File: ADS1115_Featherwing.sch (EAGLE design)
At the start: 25 parts, among them J1 4P-SMD-2.0-90D, J2 ST-PJ-312, U1 ADS1115IDGST

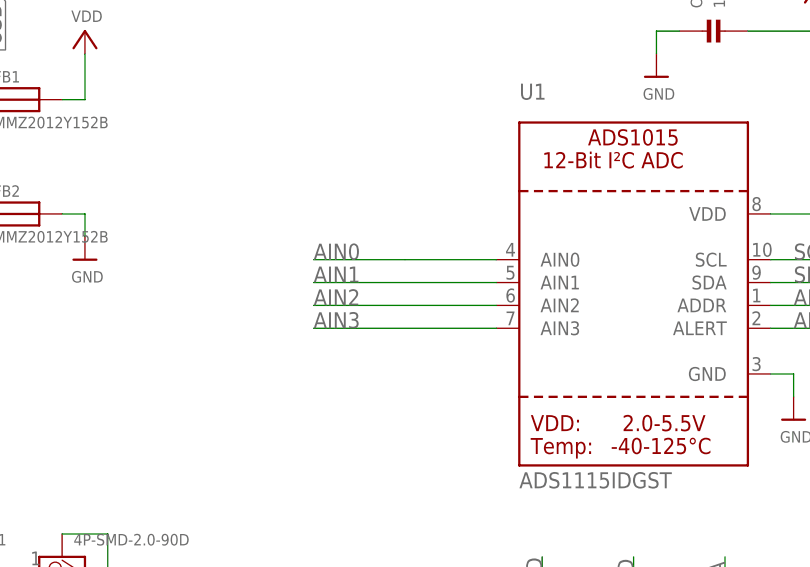
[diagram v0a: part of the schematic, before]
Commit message: Added protection resistor
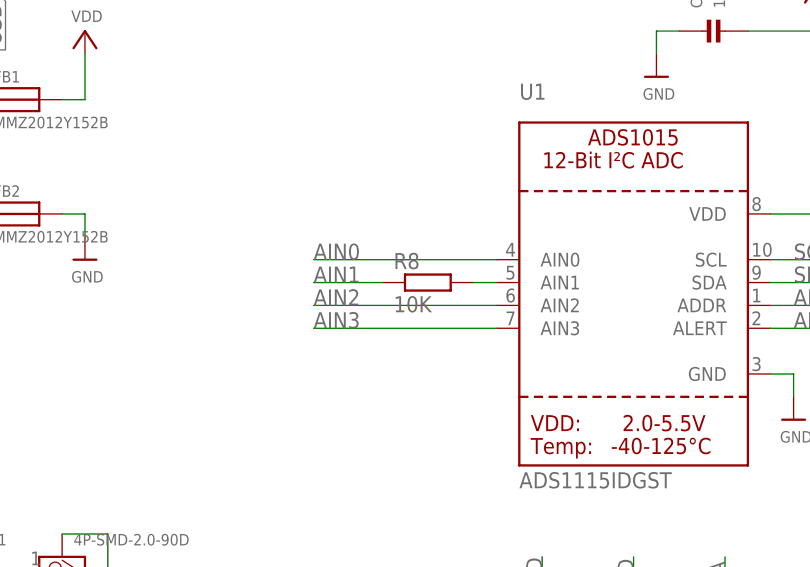
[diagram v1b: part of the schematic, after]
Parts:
- added R8: 10K, resistor:R-EU_R0603
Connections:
- new net N$1: R8.2, U1.AIN1
- net AIN1: now also R8.1; no longer U1.AIN1
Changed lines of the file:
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@@
 <?xml version="1.0" encoding="utf-8"?>
 <!DOCTYPE eagle SYSTEM "eagle.dtd">
-<eagle version="7.1.0">
+<eagle version="7.4.0">
 <drawing>
 <settings>
@@
 <grid distance="0.1" unitdist="inch" unit="inch" style="lines" multiple="1" display="no" altdistance="0.01" altunitdist="inch" altunit="inch"/>
 <layers>
-<layer number="1" name="Top" color="4" fill="1" visible="yes" active="no"/>
-<layer number="16" name="Bottom" color="1" fill="1" visible="yes" active="no"/>
-<layer number="17" name="Pads" color="2" fill="1" visible="yes" active="no"/>
-<layer number="18" name="Vias" color="2" fill="1" visible="yes" active="no"/>
-<layer number="19" name="Unrouted" color="6" fill="1" visible="yes" active="no"/>
-<layer number="20" name="Dimension" color="15" fill="1" visible="yes" active="no"/>
-<layer number="21" name="tPlace" color="7" fill="1" visible="yes" active="no"/>
-<layer number="22" name="bPlace" color="11" fill="1" visible="yes" active="no"/>
-<layer number="23" name="tOrigins" color="15" fill="1" visible="yes" active="no"/>
-<layer number="24" name="bOrigins" color="15" fill="1" visible="yes" active="no"/>
-<layer number="25" name="tNames" color="7" fill="1" visible="yes" active="no"/>
-<layer number="26" name="bNames" color="11" fill="1" visible="yes" active="no"/>
-<layer number="27" name="tValues" color="7" fill="1" visible="yes" active="no"/>
-<layer number="28" name="bValues" color="7" fill="1" visible="yes" active="no"/>
+<layer number="1" name="Top" color="4" fill="1" visible="no" active="no"/>
+<layer number="16" name="Bottom" color="1" fill="1" visible="no" active="no"/>
+<layer number="17" name="Pads" color="2" fill="1" visible="no" active="no"/>
+<layer number="18" name="Vias" color="2" fill="1" visible="no" active="no"/>
+<layer number="19" name="Unrouted" color="6" fill="1" visible="no" active="no"/>
+<layer number="20" name="Dimension" color="15" fill="1" visible="no" active="no"/>
+<layer number="21" name="tPlace" color="7" fill="1" visible="no" active="no"/>
+<layer number="22" name="bPlace" color="11" fill="1" visible="no" active="no"/>
+<layer number="23" name="tOrigins" color="15" fill="1" visible="no" active="no"/>
+<layer number="24" name="bOrigins" color="15" fill="1" visible="no" active="no"/>
+<layer number="25" name="tNames" color="7" fill="1" visible="no" active="no"/>
+<layer number="26" name="bNames" color="11" fill="1" visible="no" active="no"/>
+<layer number="27" name="tValues" color="7" fill="1" visible="no" active="no"/>
+<layer number="28" name="bValues" color="7" fill="1" visible="no" active="no"/>
 <layer number="29" name="tStop" color="7" fill="3" visible="no" active="no"/>
 <layer number="30" name="bStop" color="7" fill="6" visible="no" active="no"/>
@@
 <layer number="35" name="tGlue" color="7" fill="4" visible="no" active="no"/>
 <layer number="36" name="bGlue" color="7" fill="5" visible="no" active="no"/>
-<layer number="37" name="tTest" color="7" fill="1" visible="yes" active="no"/>
-<layer number="38" name="bTest" color="7" fill="1" visible="yes" active="no"/>
+<layer number="37" name="tTest" color="7" fill="1" visible="no" active="no"/>
+<layer number="38" name="bTest" color="7" fill="1" visible="no" active="no"/>
 <layer number="39" name="tKeepout" color="4" fill="11" visible="no" active="no"/>
 <layer number="40" name="bKeepout" color="1" fill="11" visible="no" active="no"/>
@@
 <layer number="44" name="Drills" color="7" fill="1" visible="no" active="no"/>
 <layer number="45" name="Holes" color="7" fill="1" visible="no" active="no"/>
-<layer number="46" name="Milling" color="3" fill="1" visible="yes" active="no"/>
-<layer number="47" name="Measures" color="7" fill="1" visible="yes" active="no"/>
-<layer number="48" name="Document" color="7" fill="1" visible="yes" active="no"/>
-<layer number="49" name="Reference" color="7" fill="1" visible="yes" active="no"/>
-<layer number="50" name="dxf" color="7" fill="1" visible="yes" active="no"/>
-<layer number="51" name="tDocu" color="7" fill="1" visible="yes" active="no"/>
-<layer number="52" name="bDocu" color="7" fill="1" visible="yes" active="no"/>
-<layer number="53" name="tGND_GNDA" color="7" fill="9" visible="yes" active="no"/>
-<layer number="54" name="bGND_GNDA" color="1" fill="9" visible="yes" active="no"/>
-<layer number="56" name="wert" color="7" fill="1" visible="yes" active="no"/>
-<layer number="57" name="tCAD" color="7" fill="1" visible="yes" active="no"/>
-<layer number="59" name="tCarbon" color="7" fill="1" visible="yes" active="no"/>
-<layer number="60" name="bCarbon" color="7" fill="1" visible="yes" active="no"/>
+<layer number="46" name="Milling" color="3" fill="1" visible="no" active="no"/>
+<layer number="47" name="Measures" color="7" fill="1" visible="no" active="no"/>
+<layer number="48" name="Document" color="7" fill="1" visible="no" active="no"/>
+<layer number="49" name="Reference" color="7" fill="1" visible="no" active="no"/>
+<layer number="50" name="dxf" color="7" fill="1" visible="no" active="no"/>
+<layer number="51" name="tDocu" color="7" fill="1" visible="no" active="no"/>
+<layer number="52" name="bDocu" color="7" fill="1" visible="no" active="no"/>
+<layer number="53" name="tGND_GNDA" color="7" fill="9" visible="no" active="no"/>
+<layer number="54" name="bGND_GNDA" color="1" fill="9" visible="no" active="no"/>
+<layer number="56" name="wert" color="7" fill="1" visible="no" active="no"/>
+<layer number="57" name="tCAD" color="7" fill="1" visible="no" active="no"/>
+<layer number="59" name="tCarbon" color="7" fill="1" visible="no" active="no"/>
+<layer number="60" name="bCarbon" color="7" fill="1" visible="no" active="no"/>
 <layer number="90" name="Modules" color="5" fill="1" visible="yes" active="yes"/>
 <layer number="91" name="Nets" color="2" fill="1" visible="yes" active="yes"/>
@@
 <part name="J1" library="Seeed-OPL-Connector" deviceset="GROVE-CONNECTOR-SMD-90D(4+2P-2.0)" device="" value="4P-SMD-2.0-90D"/>
 <part name="C5" library="adafruit" deviceset="CPOL-US" device="153CLV-0810" value="100uF 50V"/>
+<part name="R8" library="resistor" deviceset="R-EU_" device="R0603" value="10K"/>
 </parts>
 <sheets>
@@
 <instance part="J1" gate="G$1" x="-12.7" y="7.62"/>
 <instance part="C5" gate="G$1" x="101.6" y="114.3"/>
+<instance part="R8" gate="G$1" x="27.94" y="43.18"/>
 </instances>
 <busses>
@@
 <net name="AIN0" class="1">
 <segment>
+<label x="15.24" y="45.72" size="1.778" layer="95"/>
+<wire x1="15.24" y1="45.72" x2="35.56" y2="45.72" width="0.1524" layer="91"/>
 <pinref part="U1" gate="G$1" pin="AIN0"/>
-<wire x1="35.56" y1="45.72" x2="25.4" y2="45.72" width="0.1524" layer="91"/>
-<label x="15.24" y="45.72" size="1.778" layer="95"/>
-<wire x1="25.4" y1="45.72" x2="15.24" y2="45.72" width="0.1524" layer="91"/>
 </segment>
 <segment>
@@
 <net name="AIN1" class="0">
 <segment>
-<pinref part="U1" gate="G$1" pin="AIN1"/>
-<wire x1="35.56" y1="43.18" x2="15.24" y2="43.18" width="0.1524" layer="91"/>
-<label x="15.24" y="43.18" size="1.778" layer="95"/>
-</segment>
-<segment>
 <wire x1="-43.18" y1="35.56" x2="-27.94" y2="35.56" width="0.1524" layer="91"/>
 <label x="-38.1" y="35.56" size="1.778" layer="95"/>
@@
 <junction x="139.7" y="114.3"/>
 <label x="132.08" y="114.3" size="1.778" layer="95"/>
+</segment>
+<segment>
+<pinref part="R8" gate="G$1" pin="1"/>
+<wire x1="22.86" y1="43.18" x2="15.24" y2="43.18" width="0.1524" layer="91"/>
+<label x="15.24" y="43.18" size="1.778" layer="95"/>
 </segment>
 </net>
@@
 </segment>
 </net>
+<net name="N$1" class="0">
+<segment>
+<pinref part="U1" gate="G$1" pin="AIN1"/>
+<pinref part="R8" gate="G$1" pin="2"/>
+<wire x1="35.56" y1="43.18" x2="33.02" y2="43.18" width="0.1524" layer="91"/>
+</segment>
+</net>
